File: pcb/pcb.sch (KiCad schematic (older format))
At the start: 17 parts, among them J1 Barrel_Jack, J2 Barrel_Jack, J3 Screw_Terminal_01x02, J4 Screw_Terminal_01x02, J5 Conn_02x05_Odd_Even, J6 Conn_01x06_Male, SW1 SW_SPDT, U1 CPC5001G

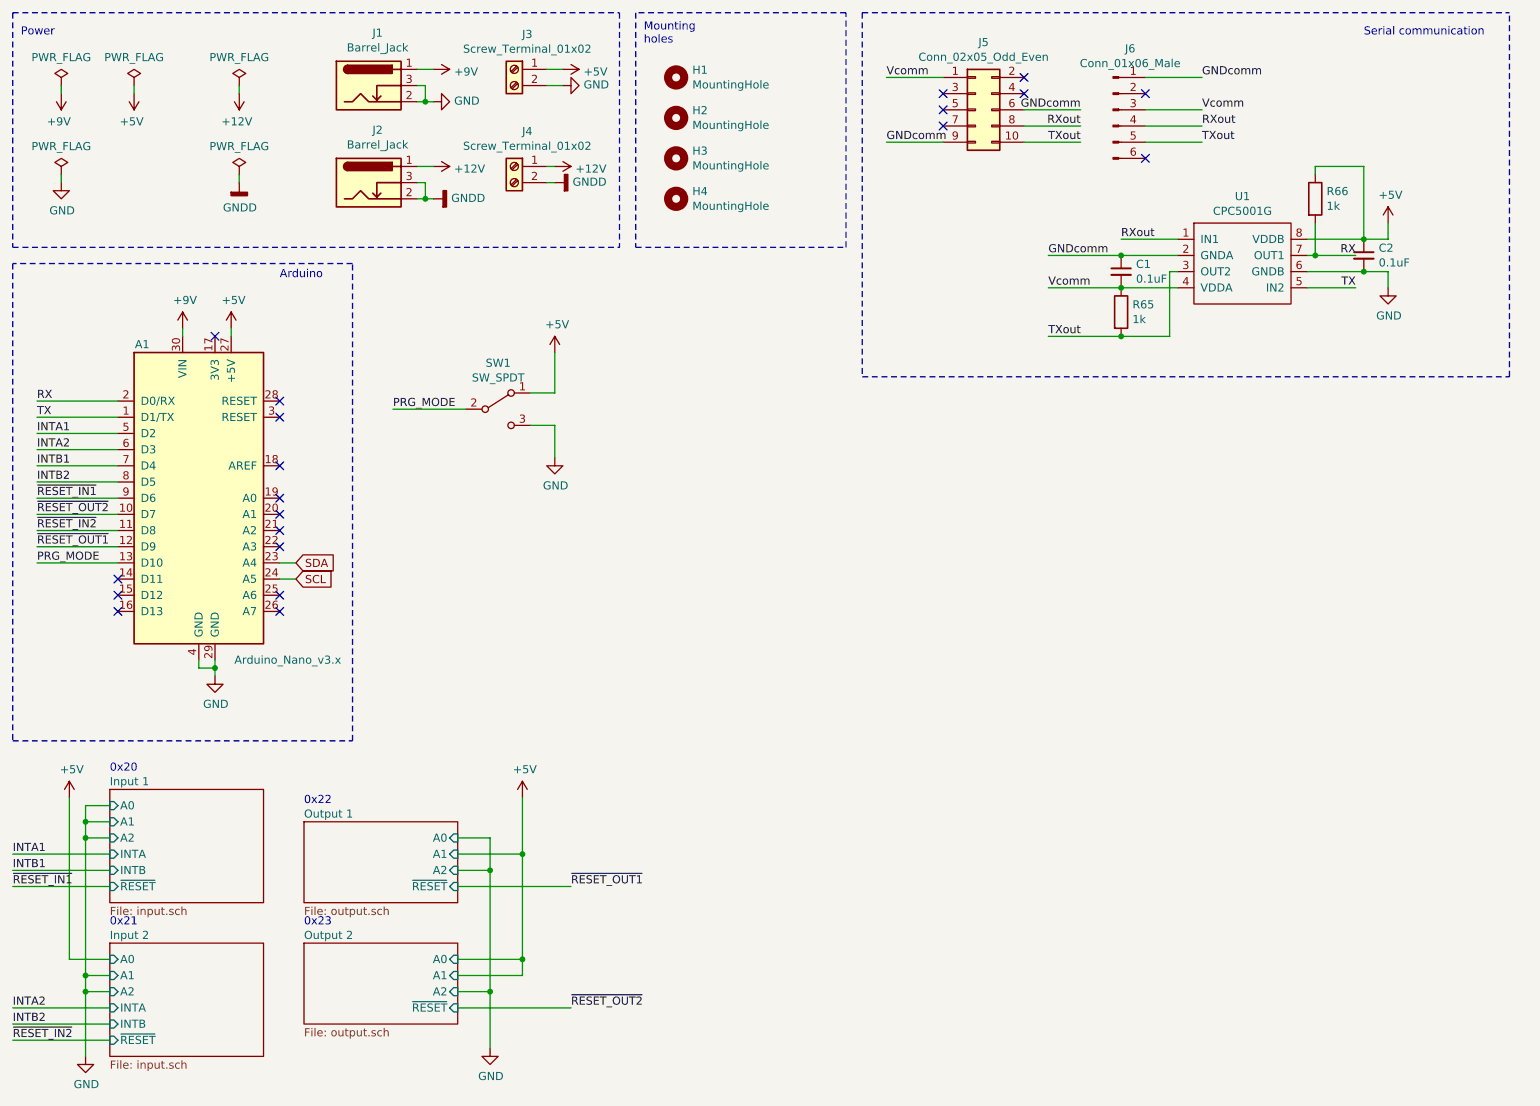
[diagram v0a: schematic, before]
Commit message: stuff
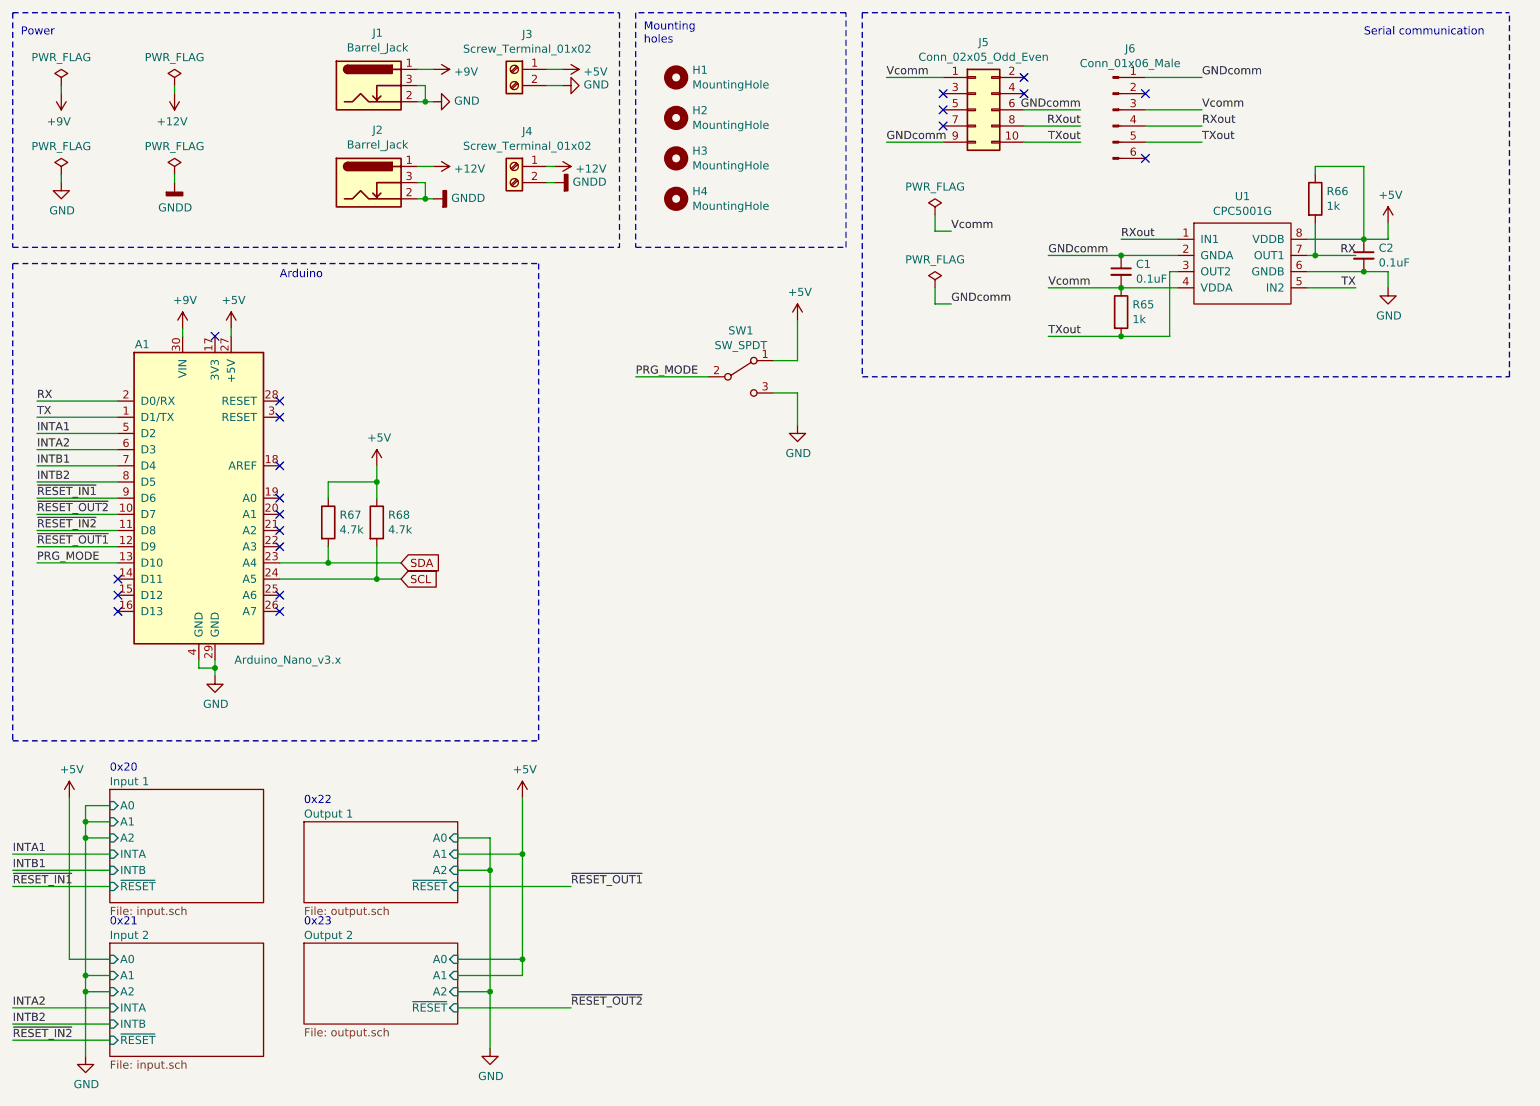
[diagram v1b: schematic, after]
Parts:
- added R67, R68: 4.7k, Resistor_THT:R_Axial_DIN0207_L6.3mm_D2.5mm_P7.62mm_Horizontal, symbol Device:R
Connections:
- net +5V: now also R67.1, R68.1
- net SCL: now also R68.2
- net SDA: now also R67.2
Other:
- moved on the sheet: SW1
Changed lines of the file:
@@
 L power:PWR_FLAG #FLG04
 U 1 1 5C20AF23
-P 2200 1300
-F 0 "#FLG04" H 2200 1375 50  0001 C CNN
-F 1 "PWR_FLAG" H 2200 1474 50  0000 C CNN
-F 2 "" H 2200 1300 50  0001 C CNN
-F 3 "~" H 2200 1300 50  0001 C CNN
-	1    2200 1300
+P 1800 1300
+F 0 "#FLG04" H 1800 1375 50  0001 C CNN
+F 1 "PWR_FLAG" H 1800 1474 50  0000 C CNN
+F 2 "" H 1800 1300 50  0001 C CNN
+F 3 "~" H 1800 1300 50  0001 C CNN
+	1    1800 1300
 	1    0    0    -1
 $EndComp
@@
 L power:PWR_FLAG #FLG05
 U 1 1 5C20AF39
-P 2200 1850
-F 0 "#FLG05" H 2200 1925 50  0001 C CNN
-F 1 "PWR_FLAG" H 2200 2024 50  0000 C CNN
-F 2 "" H 2200 1850 50  0001 C CNN
-F 3 "~" H 2200 1850 50  0001 C CNN
-	1    2200 1850
+P 1800 1850
+F 0 "#FLG05" H 1800 1925 50  0001 C CNN
+F 1 "PWR_FLAG" H 1800 2024 50  0000 C CNN
+F 2 "" H 1800 1850 50  0001 C CNN
+F 3 "~" H 1800 1850 50  0001 C CNN
+	1    1800 1850
 	1    0    0    -1
 $EndComp
@@
 	1100 1850 1100 1900
 $Comp
-L power:+5V #PWR03
-U 1 1 5C20B0FA
-P 1550 1350
-F 0 "#PWR03" H 1550 1200 50  0001 C CNN
-F 1 "+5V" H 1565 1523 50  0000 C CNN
-F 2 "" H 1550 1350 50  0001 C CNN
-F 3 "" H 1550 1350 50  0001 C CNN
-	1    1550 1350
-	-1   0    0    1
-$EndComp
-$Comp
-L power:PWR_FLAG #FLG03
-U 1 1 5C20B116
-P 1550 1300
-F 0 "#FLG03" H 1550 1375 50  0001 C CNN
-F 1 "PWR_FLAG" H 1550 1474 50  0000 C CNN
-F 2 "" H 1550 1300 50  0001 C CNN
-F 3 "~" H 1550 1300 50  0001 C CNN
-	1    1550 1300
-	1    0    0    -1
-$EndComp
-Wire Wire Line
-	1550 1300 1550 1350
-$Comp
 L power:+12V #PWR07
 U 1 1 5C20B221
-P 2200 1350
-F 0 "#PWR07" H 2200 1200 50  0001 C CNN
-F 1 "+12V" H 2215 1523 50  0000 C CNN
-F 2 "" H 2200 1350 50  0001 C CNN
-F 3 "" H 2200 1350 50  0001 C CNN
-	1    2200 1350
+P 1800 1350
+F 0 "#PWR07" H 1800 1200 50  0001 C CNN
+F 1 "+12V" H 1815 1523 50  0000 C CNN
+F 2 "" H 1800 1350 50  0001 C CNN
+F 3 "" H 1800 1350 50  0001 C CNN
+	1    1800 1350
 	-1   0    0    1
 $EndComp
@@
 L power:GNDD #PWR08
 U 1 1 5C20B289
-P 2200 1900
-F 0 "#PWR08" H 2200 1650 50  0001 C CNN
-F 1 "GNDD" H 2204 1745 50  0000 C CNN
-F 2 "" H 2200 1900 50  0001 C CNN
-F 3 "" H 2200 1900 50  0001 C CNN
-	1    2200 1900
-	1    0    0    -1
-$EndComp
-Wire Wire Line
-	2200 1300 2200 1350
-Wire Wire Line
-	2200 1850 2200 1900
+P 1800 1900
+F 0 "#PWR08" H 1800 1650 50  0001 C CNN
+F 1 "GNDD" H 1804 1745 50  0000 C CNN
+F 2 "" H 1800 1900 50  0001 C CNN
+F 3 "" H 1800 1900 50  0001 C CNN
+	1    1800 1900
+	1    0    0    -1
+$EndComp
+Wire Wire Line
+	1800 1300 1800 1350
+Wire Wire Line
+	1800 1850 1800 1900
 $Comp
 L power:GND #PWR05
@@
 NoConn ~ 2450 4450
 NoConn ~ 2450 4550
-Text GLabel 2550 4250 2    50   Input ~ 0
+Text GLabel 3200 4250 2    50   Input ~ 0
 SDA
-Text GLabel 2550 4350 2    50   Input ~ 0
+Text GLabel 3200 4350 2    50   Input ~ 0
 SCL
-Wire Wire Line
-	2450 4250 2550 4250
-Wire Wire Line
-	2550 4350 2450 4350
 $Comp
 L Connector:Barrel_Jack_Switch J1
@@
 Text Notes 2600 6500 0    50   ~ 0
 0x23
-Wire Notes Line
-	800  5350 2900 5350
-Wire Notes Line
-	2900 5350 2900 2400
-Wire Notes Line
-	2900 2400 800  2400
 Wire Wire Line
 	3300 1300 3350 1300
@@
 	3350 2000 3300 2000
 Wire Wire Line
-	4000 3400 4150 3400
-Wire Wire Line
-	4150 3400 4150 3600
+	5500 3200 5650 3200
+Wire Wire Line
+	5650 3200 5650 3400
 $Comp
 L power:GND #PWR0102
 U 1 1 5C298323
-P 4150 3600
-F 0 "#PWR0102" H 4150 3350 50  0001 C CNN
-F 1 "GND" H 4155 3427 50  0000 C CNN
-F 2 "" H 4150 3600 50  0001 C CNN
-F 3 "" H 4150 3600 50  0001 C CNN
-	1    4150 3600
-	1    0    0    -1
-$EndComp
-Text Label 3150 3300 0    50   ~ 0
+P 5650 3400
+F 0 "#PWR0102" H 5650 3150 50  0001 C CNN
+F 1 "GND" H 5655 3227 50  0000 C CNN
+F 2 "" H 5650 3400 50  0001 C CNN
+F 3 "" H 5650 3400 50  0001 C CNN
+	1    5650 3400
+	1    0    0    -1
+$EndComp
+Text Label 4650 3100 0    50   ~ 0
 PRG_MODE
 Wire Wire Line
@@
 PRG_MODE
 Wire Wire Line
-	3150 3300 3600 3300
+	4650 3100 5100 3100
 $Comp
 L Switch:SW_SPDT SW1
 U 1 1 5C2A8AB1
-P 3800 3300
-F 0 "SW1" H 3800 3585 50  0000 C CNN
-F 1 "SW_SPDT" H 3800 3494 50  0000 C CNN
-F 2 "digikey-footprints:Switch_Slide_11.6x4mm_EG1218" H 3800 3300 50  0001 C CNN
-F 3 "" H 3800 3300 50  0001 C CNN
-	1    3800 3300
+P 5300 3100
+F 0 "SW1" H 5300 3385 50  0000 C CNN
+F 1 "SW_SPDT" H 5300 3294 50  0000 C CNN
+F 2 "digikey-footprints:Switch_Slide_11.6x4mm_EG1218" H 5300 3100 50  0001 C CNN
+F 3 "" H 5300 3100 50  0001 C CNN
+	1    5300 3100
 	1    0    0    -1
 $EndComp
@@
 L power:+5V #PWR0101
 U 1 1 5C2AB353
-P 4150 2950
-F 0 "#PWR0101" H 4150 2800 50  0001 C CNN
-F 1 "+5V" H 4165 3123 50  0000 C CNN
-F 2 "" H 4150 2950 50  0001 C CNN
-F 3 "" H 4150 2950 50  0001 C CNN
-	1    4150 2950
-	1    0    0    -1
-$EndComp
-Wire Wire Line
-	4000 3200 4150 3200
-Wire Wire Line
-	4150 3200 4150 2950
+P 5650 2750
+F 0 "#PWR0101" H 5650 2600 50  0001 C CNN
+F 1 "+5V" H 5665 2923 50  0000 C CNN
+F 2 "" H 5650 2750 50  0001 C CNN
+F 3 "" H 5650 2750 50  0001 C CNN
+	1    5650 2750
+	1    0    0    -1
+$EndComp
+Wire Wire Line
+	5500 3000 5650 3000
+Wire Wire Line
+	5650 3000 5650 2750
 $Comp
 L Connector_Generic:Conn_02x05_Odd_Even J5
@@
 	-1   0    0    -1
 $EndComp
+$Comp
+L power:PWR_FLAG #FLG0101
+U 1 1 5C3B9CC1
+P 6500 2100
+F 0 "#FLG0101" H 6500 2175 50  0001 C CNN
+F 1 "PWR_FLAG" H 6500 2274 50  0000 C CNN
+F 2 "" H 6500 2100 50  0001 C CNN
+F 3 "~" H 6500 2100 50  0001 C CNN
+	1    6500 2100
+	1    0    0    -1
+$EndComp
+$Comp
+L power:PWR_FLAG #FLG0102
+U 1 1 5C3B9D55
+P 6500 2550
+F 0 "#FLG0102" H 6500 2625 50  0001 C CNN
+F 1 "PWR_FLAG" H 6500 2724 50  0000 C CNN
+F 2 "" H 6500 2550 50  0001 C CNN
+F 3 "~" H 6500 2550 50  0001 C CNN
+	1    6500 2550
+	1    0    0    -1
+$EndComp
+Wire Wire Line
+	6500 2100 6500 2200
+Wire Wire Line
+	6500 2200 6600 2200
+Wire Wire Line
+	6500 2550 6500 2650
+Wire Wire Line
+	6500 2650 6600 2650
+Text Label 6600 2200 0    50   ~ 0
+Vcomm
+Text Label 6600 2650 0    50   ~ 0
+GNDcomm
+Wire Notes Line
+	4050 2400 4050 5350
+Wire Notes Line
+	800  5350 4050 5350
+Wire Notes Line
+	800  2400 4050 2400
+Wire Wire Line
+	2450 4250 2750 4250
+Wire Wire Line
+	2450 4350 3050 4350
+$Comp
+L Device:R R67
+U 1 1 5C3D4A20
+P 2750 4000
+F 0 "R67" H 2820 4046 50  0000 L CNN
+F 1 "4.7k" H 2820 3955 50  0000 L CNN
+F 2 "Resistor_THT:R_Axial_DIN0207_L6.3mm_D2.5mm_P7.62mm_Horizontal" V 2680 4000 50  0001 C CNN
+F 3 "~" H 2750 4000 50  0001 C CNN
+	1    2750 4000
+	1    0    0    -1
+$EndComp
+$Comp
+L Device:R R68
+U 1 1 5C3D4A7A
+P 3050 4000
+F 0 "R68" H 3120 4046 50  0000 L CNN
+F 1 "4.7k" H 3120 3955 50  0000 L CNN
+F 2 "Resistor_THT:R_Axial_DIN0207_L6.3mm_D2.5mm_P7.62mm_Horizontal" V 2980 4000 50  0001 C CNN
+F 3 "~" H 3050 4000 50  0001 C CNN
+	1    3050 4000
+	1    0    0    -1
+$EndComp
+Wire Wire Line
+	2750 4150 2750 4250
+Connection ~ 2750 4250
+Wire Wire Line
+	2750 4250 3200 4250
+Wire Wire Line
+	3050 4150 3050 4350
+Connection ~ 3050 4350
+Wire Wire Line
+	3050 4350 3200 4350
+Wire Wire Line
+	2750 3850 2750 3750
+Wire Wire Line
+	2750 3750 3050 3750
+Wire Wire Line
+	3050 3750 3050 3850
+Wire Wire Line
+	3050 3750 3050 3650
+Connection ~ 3050 3750
+$Comp
+L power:+5V #PWR0105
+U 1 1 5C3E2C4F
+P 3050 3650
+F 0 "#PWR0105" H 3050 3500 50  0001 C CNN
+F 1 "+5V" H 3065 3823 50  0000 C CNN
+F 2 "" H 3050 3650 50  0001 C CNN
+F 3 "" H 3050 3650 50  0001 C CNN
+	1    3050 3650
+	1    0    0    -1
+$EndComp
 $EndSCHEMATC
